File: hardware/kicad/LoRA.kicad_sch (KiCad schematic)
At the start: 0 parts

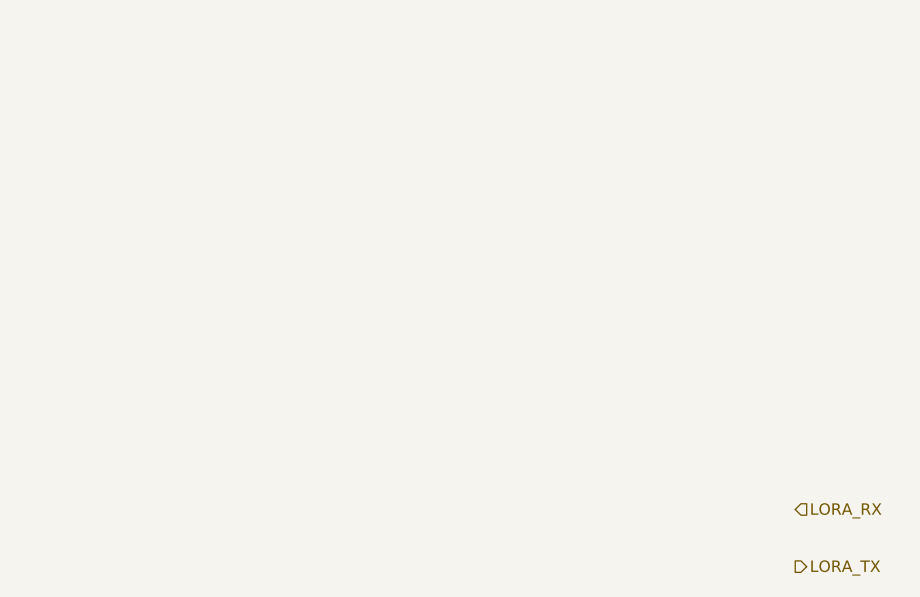
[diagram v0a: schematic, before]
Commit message: GPS and LoRA completed
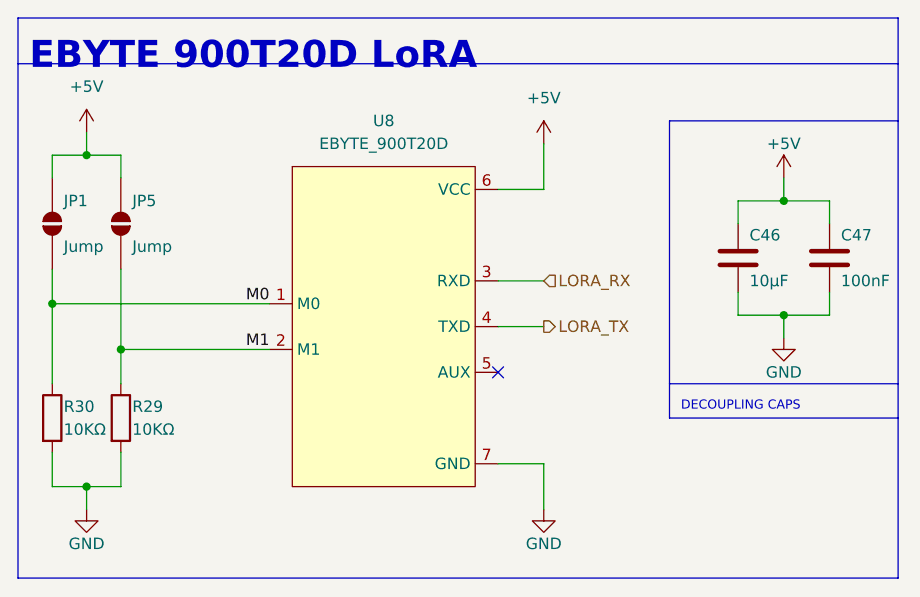
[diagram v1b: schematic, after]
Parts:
- added C46: 10μF, symbol Device:C
- added C47: 100nF, symbol Device:C
- added JP1, JP5: Jump, symbol Jumper:SolderJumper_2_Open
- added R29, R30: 10KΩ, symbol Device:R
- added U8: EBYTE_900T20D, EBYTE_900T20D:EBYTE_900T20D, symbol EBYTE_900T20D:EBYTE_900T20D
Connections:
- net LORA_RX: now also U8.3 (RXD)
- net LORA_TX: now also U8.4 (TXD)
- new net: U8.10 (NC), U8.8 (NC), U8.9 (NC)
- new net +5V: C46.1, C47.1, JP1.2 (B), JP5.2 (B), U8.6 (VCC)
- new net GND: C46.2, C47.2, R29.2, R30.2, U8.7 (GND)
- new net M0: JP1.1 (A), R30.1, U8.1 (M0)
- new net M1: JP5.1 (A), R29.1, U8.2 (M1)
- no-connect marks 0 -> 1
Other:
- note added: "DECOUPLING CAPS"
- note added: "EBYTE 900T20D LoRA"
